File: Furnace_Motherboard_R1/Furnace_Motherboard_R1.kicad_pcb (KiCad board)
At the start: 2 copper layers, 13 parts, among them U1 STM32H563VITx

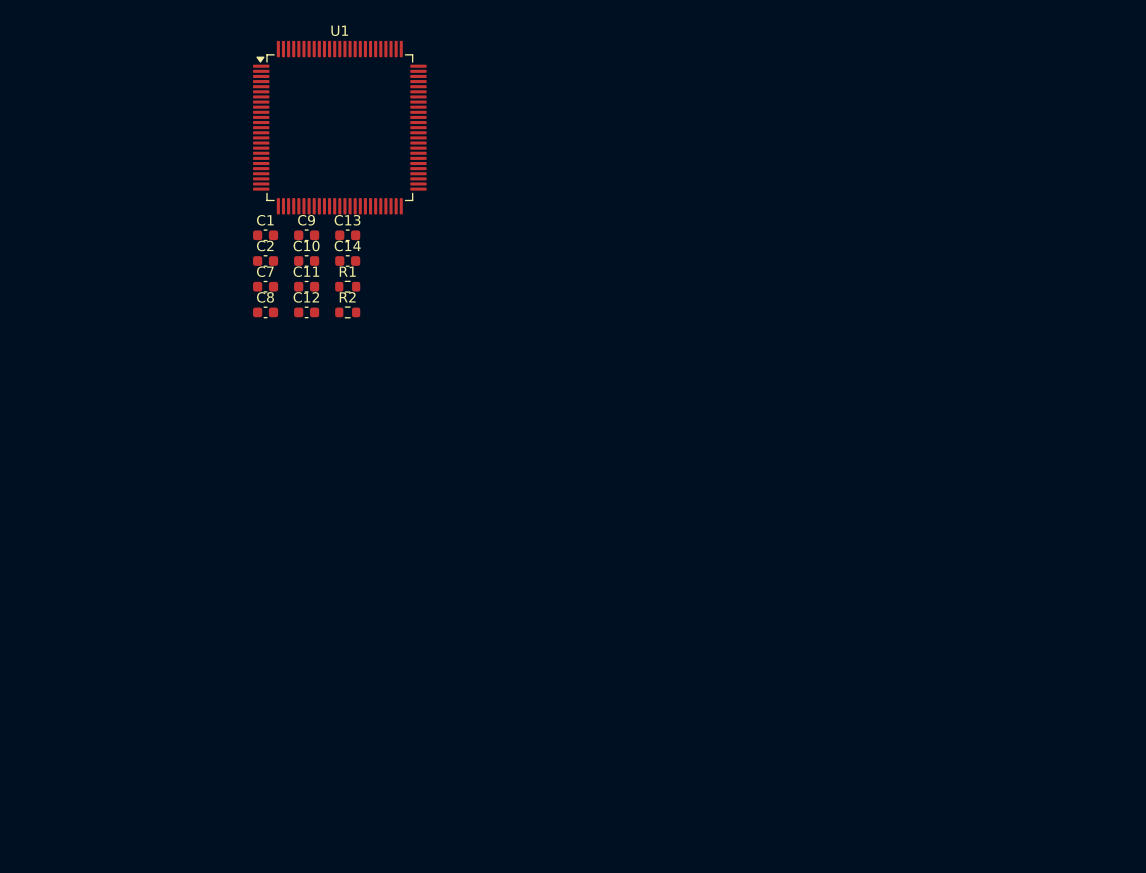
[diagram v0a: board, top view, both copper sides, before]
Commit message: Back up motherboard R1 design and fabrication outputs
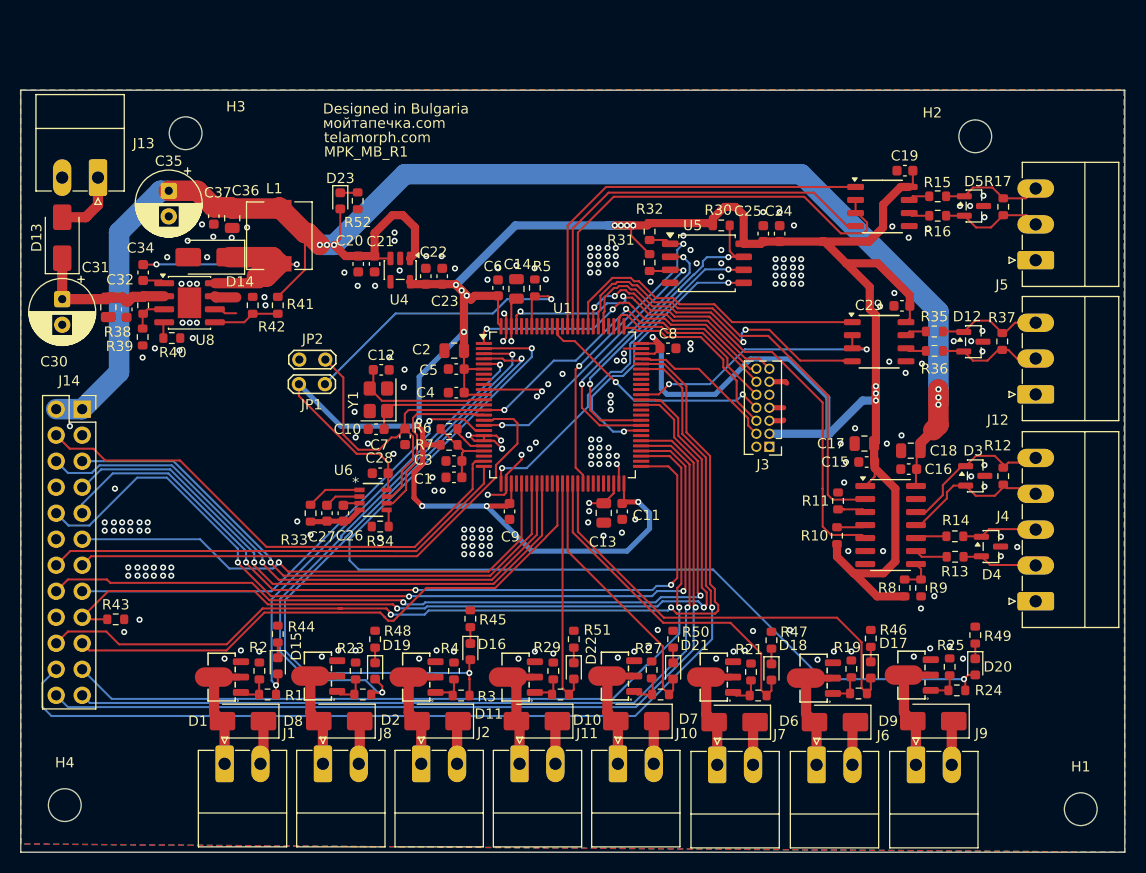
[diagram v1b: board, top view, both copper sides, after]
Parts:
- added C15: 100n, Capacitor_SMD:C_0603_1608Metric, F.Cu at (134.4, 93.1)
- added C16: 100n, Capacitor_SMD:C_0603_1608Metric, F.Cu at (138.5, 93.8)
- added C17: 1u, Capacitor_SMD:C_0805_2012Metric, F.Cu at (134.2, 91.3)
- added C18: 1u, Capacitor_SMD:C_0805_2012Metric, F.Cu at (138.7, 92.0)
- added C19: 100n, Capacitor_SMD:C_0603_1608Metric, F.Cu at (138.1, 64.7)
- added C20: 1u, Capacitor_SMD:C_0603_1608Metric, F.Cu at (84.8, 73.8)
- added C21: 100n, Capacitor_SMD:C_0603_1608Metric, F.Cu at (86.3, 73.8)
- added C22: 100n, Capacitor_SMD:C_0603_1608Metric, F.Cu at (91.3, 75.0)
- added C23: 1u, Capacitor_SMD:C_0603_1608Metric, F.Cu at (93.0, 75.0)
- added C24: 1u, Capacitor_SMD:C_0603_1608Metric, F.Cu at (125.9, 70.8)
- added C25: 100n, Capacitor_SMD:C_0603_1608Metric, F.Cu at (124.3, 70.8)
- added C26: 22n, Capacitor_SMD:C_0603_1608Metric, F.Cu at (83.3, 98.1)
- added C27: 3.3n, Capacitor_SMD:C_0603_1608Metric, F.Cu at (81.7, 98.1)
- added C28: 100n, Capacitor_SMD:C_0603_1608Metric, F.Cu at (86.9, 94.2)
- added C29: 100n, Capacitor_SMD:C_0603_1608Metric, F.Cu at (137.8, 77.9)
- added C3: 1u, Capacitor_SMD:C_0603_1608Metric, F.Cu at (94.1, 93.0)
- added C30: 47u, Capacitor_THT:CP_Radial_D6.3mm_P2.50mm, F.Cu at (55.9, 77.2)
- added C31: 2.2u, Capacitor_SMD:C_0805_2012Metric, F.Cu at (60.4, 78.0)
- added C32: 100n, Capacitor_SMD:C_0603_1608Metric, F.Cu at (62.1, 78.2)
- added C34: 100n, Capacitor_SMD:C_0603_1608Metric, F.Cu at (63.8, 74.6)
- added C35: 47u, Capacitor_THT:CP_Radial_D6.3mm_P2.50mm, F.Cu at (66.2, 66.6)
- added C36: 10u, Capacitor_SMD:C_0805_2012Metric, F.Cu at (72.5, 69.3)
- added C37: 100n, Capacitor_SMD:C_0603_1608Metric, F.Cu at (70.7, 69.1)
- added C4: 100n, Capacitor_SMD:C_0603_1608Metric, F.Cu at (94.3, 86.3)
- added C5: 100n, Capacitor_SMD:C_0603_1608Metric, F.Cu at (94.3, 84.0)
- added C6: 100n, Capacitor_SMD:C_0603_1608Metric, F.Cu at (98.4, 76.1)
- added D1: US1B, Diode_SMD:D_SMA, F.Cu at (73.5, 118.4)
- added D10: US1B, Diode_SMD:D_SMA, F.Cu at (111.9, 118.4)
- added D11: US1B, Diode_SMD:D_SMA, F.Cu at (102.2, 118.4)
- added D12: SM712_SOT23, Package_TO_SOT_SMD:SOT-23, F.Cu at (144.8, 81.4)
- added D13: SS36, Diode_SMD:D_SMA, F.Cu at (55.9, 71.2)
- added D14: SS36, Diode_SMD:D_SMA, F.Cu at (70.2, 73.1)
- added D15: LED, LED_SMD:LED_0603_1608Metric, F.Cu at (76.9, 113.0)
- added D16: LED, LED_SMD:LED_0603_1608Metric, F.Cu at (95.7, 111.6)
- added D17: LED, LED_SMD:LED_0603_1608Metric, F.Cu at (134.8, 113.4)
- added D18: LED, LED_SMD:LED_0603_1608Metric, F.Cu at (125.1, 113.6)
- added D19: LED, LED_SMD:LED_0603_1608Metric, F.Cu at (86.4, 113.5)
- added D2: US1B, Diode_SMD:D_SMA, F.Cu at (92.5, 118.4)
- added D20: LED, LED_SMD:LED_0603_1608Metric, F.Cu at (145.0, 113.1)
- added D21: LED, LED_SMD:LED_0603_1608Metric, F.Cu at (115.5, 113.5)
- added D22: LED, LED_SMD:LED_0603_1608Metric, F.Cu at (105.8, 113.5)
- added D23: LED, LED_SMD:LED_0603_1608Metric, F.Cu at (83.0, 67.6)
- added D3: SM712_SOT23, Package_TO_SOT_SMD:SOT-23, F.Cu at (145.0, 94.5)
- added D4: SM712_SOT23, Package_TO_SOT_SMD:SOT-23, F.Cu at (146.5, 101.4)
- added D5: SM712_SOT23, Package_TO_SOT_SMD:SOT-23, F.Cu at (144.9, 68.1)
- added D6: US1B, Diode_SMD:D_SMA, F.Cu at (131.3, 118.5)
- added D7: US1B, Diode_SMD:D_SMA, F.Cu at (121.5, 118.5)
- added D8: US1B, Diode_SMD:D_SMA, F.Cu at (82.9, 118.4)
- added D9: US1B, Diode_SMD:D_SMA, F.Cu at (140.9, 118.4)
- added H1: MountingHole, MountingHole:MountingHole_3.2mm_M3, F.Cu at (155.3, 127.0)
- added H2: MountingHole, MountingHole:MountingHole_3.2mm_M3, F.Cu at (145.0, 61.3)
- added H3: MountingHole, MountingHole:MountingHole_3.2mm_M3, F.Cu at (67.9, 61.0)
- added H4: MountingHole, MountingHole:MountingHole_3.2mm_M3, F.Cu at (56.1, 126.6)
- added J1: Conn_01x02, Connector_Phoenix_MC:PhoenixContact_MC_1,5_2-G-3.5_1x02_P3.50mm_Horizontal, F.Cu at (71.7, 122.6)
- added J10: Conn_01x02, Connector_Phoenix_MC:PhoenixContact_MC_1,5_2-G-3.5_1x02_P3.50mm_Horizontal, F.Cu at (110.1, 122.6)
- added J11: Conn_01x02, Connector_Phoenix_MC:PhoenixContact_MC_1,5_2-G-3.5_1x02_P3.50mm_Horizontal, F.Cu at (100.5, 122.6)
- added J12: Conn_01x03, Connector_Phoenix_MC:PhoenixContact_MC_1,5_3-G-3.5_1x03_P3.50mm_Horizontal, F.Cu at (150.9, 86.5)
- added J13: Conn_01x02, Connector_Phoenix_MC:PhoenixContact_MC_1,5_2-G-3.5_1x02_P3.50mm_Horizontal, F.Cu at (59.3, 65.3)
- added J14: Conn_02x12_Odd_Even, Connector_PinSocket_2.54mm:PinSocket_2x12_P2.54mm_Vertical, F.Cu at (57.8, 87.9)
- added J2: Conn_01x02, Connector_Phoenix_MC:PhoenixContact_MC_1,5_2-G-3.5_1x02_P3.50mm_Horizontal, F.Cu at (90.9, 122.6)
- added J3: Conn_02x07_Odd_Even, Connector_PinHeader_1.27mm:PinHeader_2x07_P1.27mm_Vertical, F.Cu at (124.9, 91.6)
- added J4: Conn_01x05, Connector_Phoenix_MC:PhoenixContact_MC_1,5_5-G-3.5_1x05_P3.50mm_Horizontal, F.Cu at (150.9, 106.7)
- added J5: Conn_01x03, Connector_Phoenix_MC:PhoenixContact_MC_1,5_3-G-3.5_1x03_P3.50mm_Horizontal, F.Cu at (150.9, 73.4)
- added J6: Conn_01x02, Connector_Phoenix_MC:PhoenixContact_MC_1,5_2-G-3.5_1x02_P3.50mm_Horizontal, F.Cu at (129.5, 122.7)
- added J7: Conn_01x02, Connector_Phoenix_MC:PhoenixContact_MC_1,5_2-G-3.5_1x02_P3.50mm_Horizontal, F.Cu at (119.8, 122.7)
- added J8: Conn_01x02, Connector_Phoenix_MC:PhoenixContact_MC_1,5_2-G-3.5_1x02_P3.50mm_Horizontal, F.Cu at (81.3, 122.6)
- added J9: Conn_01x02, Connector_Phoenix_MC:PhoenixContact_MC_1,5_2-G-3.5_1x02_P3.50mm_Horizontal, F.Cu at (139.2, 122.7)
- added JP1: Jumper_2_Open, TestPoint:TestPoint_2Pads_Pitch2.54mm_Drill0.8mm, F.Cu at (81.5, 85.5)
- added JP2: Jumper_2_Open, TestPoint:TestPoint_2Pads_Pitch2.54mm_Drill0.8mm, F.Cu at (79.0, 83.1)
- added L1: 33u, Inductor_SMD:L_6.3x6.3_H3, F.Cu at (77.0, 71.0)
- added Q1: BSS606N, PCM_JLCPCB:Q_SOT-89, F.Cu at (72.0, 114.1)
- added Q2: BSS606N, PCM_JLCPCB:Q_SOT-89, F.Cu at (91.0, 114.1)
- added Q3: BSS606N, PCM_JLCPCB:Q_SOT-89, F.Cu at (129.8, 114.2)
- added Q4: BSS606N, PCM_JLCPCB:Q_SOT-89, F.Cu at (120.0, 114.1)
- added Q5: BSS606N, PCM_JLCPCB:Q_SOT-89, F.Cu at (81.4, 114.0)
- added Q6: BSS606N, PCM_JLCPCB:Q_SOT-89, F.Cu at (139.3, 113.9)
- added Q7: BSS606N, PCM_JLCPCB:Q_SOT-89, F.Cu at (110.4, 114.0)
- added Q8: BSS606N, PCM_JLCPCB:Q_SOT-89, F.Cu at (100.7, 114.1)
- added R10: 10k, Resistor_SMD:R_0603_1608Metric, F.Cu at (131.5, 100.3)
- added R11: 10k, Resistor_SMD:R_0603_1608Metric, F.Cu at (131.6, 96.9)
- added R12: 120, Resistor_SMD:R_0603_1608Metric, F.Cu at (147.7, 94.5)
- added R13: 15, Resistor_SMD:R_0603_1608Metric, F.Cu at (143.0, 102.4)
- added R14: 15, Resistor_SMD:R_0603_1608Metric, F.Cu at (143.0, 100.4)
- added R15: 15, Resistor_SMD:R_0603_1608Metric, F.Cu at (141.3, 67.2)
- added R16: 15, Resistor_SMD:R_0603_1608Metric, F.Cu at (141.3, 69.1)
- added R17: 120, Resistor_SMD:R_0603_1608Metric, F.Cu at (147.7, 68.2)
- added R18: 100, Resistor_SMD:R_0603_1608Metric, F.Cu at (133.6, 115.7)
- added R19: 10k, Resistor_SMD:R_0603_1608Metric, F.Cu at (132.9, 113.3)
- added R20: 100, Resistor_SMD:R_0603_1608Metric, F.Cu at (123.8, 115.9)
- added R21: 10k, Resistor_SMD:R_0603_1608Metric, F.Cu at (123.1, 113.6)
- added R22: 100, Resistor_SMD:R_0603_1608Metric, F.Cu at (85.2, 115.8)
- added R23: 10k, Resistor_SMD:R_0603_1608Metric, F.Cu at (84.5, 113.5)
- added R24: 100, Resistor_SMD:R_0603_1608Metric, F.Cu at (143.2, 115.4)
- added R25: 10k, Resistor_SMD:R_0603_1608Metric, F.Cu at (142.5, 113.1)
- added R26: 100, Resistor_SMD:R_0603_1608Metric, F.Cu at (114.3, 115.8)
- added R27: 10k, Resistor_SMD:R_0603_1608Metric, F.Cu at (113.4, 113.4)
- added R28: 100, Resistor_SMD:R_0603_1608Metric, F.Cu at (104.5, 115.8)
- added R29: 10k, Resistor_SMD:R_0603_1608Metric, F.Cu at (103.8, 113.5)
- added R3: 100, Resistor_SMD:R_0603_1608Metric, F.Cu at (94.8, 115.9)
- added R30: 10k, Resistor_SMD:R_0603_1608Metric, F.Cu at (120.2, 70.0)
- added R31: 10k, Resistor_SMD:R_0603_1608Metric, F.Cu at (113.2, 73.6)
- added R32: 10k, Resistor_SMD:R_0603_1608Metric, F.Cu at (113.2, 70.6)
- added R33: 10k, Resistor_SMD:R_0603_1608Metric, F.Cu at (80.1, 98.1)
- added R34: 10k, Resistor_SMD:R_0603_1608Metric, F.Cu at (86.9, 99.4)
- added R35: 15, Resistor_SMD:R_0603_1608Metric, F.Cu at (141.0, 80.4)
- added R36: 15, Resistor_SMD:R_0603_1608Metric, F.Cu at (141.0, 82.3)
- added R37: 120, Resistor_SMD:R_0603_1608Metric, F.Cu at (147.6, 81.3)
- added R38: 560k, Resistor_SMD:R_0603_1608Metric, F.Cu at (63.8, 77.8)
- added R39: 39k, Resistor_SMD:R_0603_1608Metric, F.Cu at (63.7, 80.9)
- added R4: 10k, Resistor_SMD:R_0603_1608Metric, F.Cu at (94.1, 113.5)
- added R40: 56k, Resistor_SMD:R_0603_1608Metric, F.Cu at (66.5, 81.0)
- added R41: 56k, Resistor_SMD:R_0603_1608Metric, F.Cu at (76.9, 77.8)
- added R42: 10k, Resistor_SMD:R_0603_1608Metric, F.Cu at (74.5, 77.8)
- added R43: 10k, Resistor_SMD:R_0603_1608Metric, F.Cu at (61.1, 108.5)
- added R44: 150, Resistor_SMD:R_0603_1608Metric, F.Cu at (76.9, 109.9)
- added R45: 150, Resistor_SMD:R_0603_1608Metric, F.Cu at (95.7, 108.4)
- added R46: 150, Resistor_SMD:R_0603_1608Metric, F.Cu at (134.8, 110.3)
- added R47: 150, Resistor_SMD:R_0603_1608Metric, F.Cu at (125.1, 110.5)
- added R48: 150, Resistor_SMD:R_0603_1608Metric, F.Cu at (86.4, 110.4)
- added R49: 150, Resistor_SMD:R_0603_1608Metric, F.Cu at (145.0, 110.0)
- added R5: 10k, Resistor_SMD:R_0603_1608Metric, F.Cu at (102.0, 76.1)
- added R50: 150, Resistor_SMD:R_0603_1608Metric, F.Cu at (115.5, 110.4)
- added R51: 150, Resistor_SMD:R_0603_1608Metric, F.Cu at (105.8, 110.4)
- added R52: 330, Resistor_SMD:R_0603_1608Metric, F.Cu at (84.7, 67.6)
- added R6: 0, Resistor_SMD:R_0603_1608Metric, F.Cu at (93.6, 89.9)
- added R7: 0, Resistor_SMD:R_0603_1608Metric, F.Cu at (93.6, 91.4)
- added R8: 10k, Resistor_SMD:R_0603_1608Metric, F.Cu at (138.1, 105.4)
- added R9: 0, Resistor_SMD:R_0603_1608Metric, F.Cu at (139.7, 105.4)
- added U2: PTHVD2452VDR, PCM_JLCPCB:SOIC-14_L8.7-W3.9-P1.27-LS6.0-BL, F.Cu at (136.7, 99.3)
- added U3: THVD2450DR, PCM_JLCPCB:SOIC-8_3.9x4.9mm_P1.27mm, F.Cu at (135.9, 68.2)
- added U4: TPS7A20xxxDBV, Package_TO_SOT_SMD:SOT-23-5, F.Cu at (88.8, 74.4)
- added U5: W25Q128JVS, Package_SO:SOIC-8_5.3x5.3mm_P1.27mm, F.Cu at (118.8, 73.7)
- added U6: TPS36BA38ACADDFRQ1, Furnace_TI:SOT-23-THIN-8_DDF_TEX, F.Cu at (86.2, 96.8)
- added U7: THVD2450DR, PCM_JLCPCB:SOIC-8_3.9x4.9mm_P1.27mm, F.Cu at (135.6, 81.4)
- added U8: LMR16030SDDAR, Package_SO:SOIC-8-1EP_3.9x4.9mm_P1.27mm_EP2.29x3mm, F.Cu at (68.3, 77.5)
- added Y1: Crystal_GND24_Small, Crystal:Crystal_SMD_3225-4Pin_3.2x2.5mm, F.Cu at (86.7, 87.0)
- C1: value 2.2u -> 100n
- C10: value 100n -> C
- C12: value 1u -> C
- C13: value 100n -> 2.2u; footprint Capacitor_SMD:C_0603_1608Metric -> Capacitor_SMD:C_0805_2012Metric
- C14: value 4.7u -> 2.2u; footprint Capacitor_SMD:C_0603_1608Metric -> Capacitor_SMD:C_0805_2012Metric
- C2: value 2.2u -> 4.7u; footprint Capacitor_SMD:C_0603_1608Metric -> Capacitor_SMD:C_0805_2012Metric
- R1: value 0 -> 100
- R2: value 0 -> 10k
- moved R1 40.6 mm to (75.9, 115.8), turned to 180 degrees
- moved C8 39.5 mm to (115.0, 82.0)
- moved C11 37.8 mm to (110.5, 97.9), turned to -90 degrees
- moved C13 36.9 mm to (108.7, 98.1), turned to -90 degrees
- moved R2 36.1 mm to (75.1, 113.5), turned to 90 degrees
- moved U1 34.7 mm to (104.7, 87.5)
- moved C9 33.5 mm to (99.5, 97.9), turned to -90 degrees
- moved C1 29.9 mm to (94.1, 94.6), turned to 180 degrees
- moved C2 20.4 mm to (94.1, 82.2), turned to 180 degrees
- moved C7 20.0 mm to (89.3, 90.6), turned to -90 degrees
- moved C10 17.8 mm to (86.5, 89.9), turned to 180 degrees
- moved C14 16.7 mm to (100.2, 76.2), turned to 90 degrees
- moved C12 9.19 mm to (87.0, 84.1)
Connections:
- C1 pad 1: Net-(C1-Pad1) -> /MAIN_MCU/VDDA
- C1 pad 2: MCU_GND -> GND
- C10 pad 1: +3V3 -> /MAIN_MCU/RCC_OSC_OUT
- C10 pad 2: MCU_GND -> GND
- C11 pad 2: MCU_GND -> GND
- C12 pad 1: +3V3 -> /MAIN_MCU/RCC_OSC_IN
- C12 pad 2: MCU_GND -> GND
- C13 pad 1: +3V3 -> Net-(C13-Pad1)
- C13 pad 2: MCU_GND -> GND
- C14 pad 1: +3V3 -> Net-(C13-Pad1)
- C14 pad 2: MCU_GND -> GND
- C2 pad 1: Net-(C2-Pad1) -> +3V3
- C2 pad 2: MCU_GND -> GND
- C7 pad 1: +3V3 -> /SUP_RESET_N
- C7 pad 2: MCU_GND -> GND
- C8 pad 2: MCU_GND -> GND
- C9 pad 2: MCU_GND -> GND
- R1 pad 1: Net-(U1-VBAT) -> /AUX_DO3_CMD
- R1 pad 2: Net-(U1-VDDA) -> Net-(Q1-G)
- R2 pad 1: +3V3 -> Net-(Q1-G)
- R2 pad 2: Net-(U1-VREF+) -> GND
- U1 pad 1: unconnected-(U1-PE2-Pad1) -> /MAIN_MCU/UART8_TX
- U1 pad 10: MCU_GND -> GND
- U1 pad 100: Net-(U1-VBAT) -> +3V3
- U1 pad 11: Net-(U1-VBAT) -> +3V3
- U1 pad 12: unconnected-(U1-PH0-Pad12) -> /MAIN_MCU/RCC_OSC_IN
- U1 pad 13: unconnected-(U1-PH1-Pad13) -> /MAIN_MCU/RCC_OSC_OUT
- U1 pad 14: unconnected-(U1-NRST-Pad14) -> /SUP_RESET_N
- U1 pad 15: unconnected-(U1-PC0-Pad15) -> /SUP_WDI
- U1 pad 16: unconnected-(U1-PC1-Pad16) -> /ETH_MDC
- U1 pad 17: unconnected-(U1-PC2-Pad17) -> /OCTOSPI1_IO2
- U1 pad 18: unconnected-(U1-PC3-Pad18) -> /ETH_PHY_RST_N
- U1 pad 19: MCU_GND -> GND
- U1 pad 2: unconnected-(U1-PE3-Pad2) -> /AUX_DO0_CMD
- U1 pad 20: MCU_GND -> GND
- U1 pad 22: Net-(U1-VDDA) -> /MAIN_MCU/VDDA
- U1 pad 24: unconnected-(U1-PA1-Pad24) -> /ETH_REF_CLK
- U1 pad 25: unconnected-(U1-PA2-Pad25) -> /ETH_MDIO
- U1 pad 26: unconnected-(U1-PA3-Pad26) -> /OCTOSPI1_CLK
- U1 pad 27: MCU_GND -> GND
- U1 pad 28: Net-(U1-VBAT) -> +3V3
- U1 pad 3: unconnected-(U1-PE4-Pad3) -> /AUX_DO1_CMD
- U1 pad 30: unconnected-(U1-PA5-Pad30) -> /ETH_TX_EN
- U1 pad 32: unconnected-(U1-PA7-Pad32) -> /ETH_CRS_DV
- U1 pad 33: unconnected-(U1-PC4-Pad33) -> /ETH_RXD0
- U1 pad 34: unconnected-(U1-PC5-Pad34) -> /ETH_RXD1
- U1 pad 37: unconnected-(U1-PB2-Pad37) -> /CAN_STB
- U1 pad 38: unconnected-(U1-PE7-Pad38) -> /AUX_DO4_CMD
- U1 pad 39: unconnected-(U1-PE8-Pad39) -> /AUX_DO5_CMD
- U1 pad 4: unconnected-(U1-PE5-Pad4) -> /AUX_DO2_CMD
- U1 pad 40: unconnected-(U1-PE9-Pad40) -> /HEATER_CONTACTOR_CMD
- U1 pad 41: unconnected-(U1-PE10-Pad41) -> /HEATER_SSR_CMD
- U1 pad 42: unconnected-(U1-PE11-Pad42) -> /OCTOSPI1_NCS
- U1 pad 48: Net-(C1-Pad1) -> Net-(C13-Pad1)
- U1 pad 49: MCU_GND -> GND
- U1 pad 5: unconnected-(U1-PE6-Pad5) -> /AUX_DO3_CMD
- U1 pad 51: unconnected-(U1-PB12-Pad51) -> /ETH_TXD0
- U1 pad 53: unconnected-(U1-PB14-Pad53) -> /EXT_RS485_DE
- U1 pad 54: unconnected-(U1-PB15-Pad54) -> /ETH_TXD1
- U1 pad 55: unconnected-(U1-PD8-Pad55) -> /EXT_RS485_TX
- U1 pad 56: unconnected-(U1-PD9-Pad56) -> /EXT_RS485_RX
- U1 pad 58: unconnected-(U1-PD11-Pad58) -> /OCTOSPI1_IO0
- U1 pad 59: unconnected-(U1-PD12-Pad59) -> /OCTOSPI1_IO1
- U1 pad 6: Net-(U1-VBAT) -> +3V3
- U1 pad 60: unconnected-(U1-PD13-Pad60) -> /OCTOSPI1_IO3
- U1 pad 63: unconnected-(U1-PC6-Pad63) -> /ETH_PHY_INT_N
- U1 pad 64: unconnected-(U1-PC7-Pad64) -> /ETH_MODULE_PRESENT
- U1 pad 65: unconnected-(U1-PC8-Pad65) -> /AUX_RS485_DE
- U1 pad 70: unconnected-(U1-PA11-Pad70) -> /FDCAN1_RX
- U1 pad 71: unconnected-(U1-PA12-Pad71) -> /FDCAN1_TX
- U1 pad 72: unconnected-(U1-PA13(JTMS-Pad72) -> /MAIN_MCU/DEBUG_JTMS-SWDIO
- U1 pad 73: Net-(U1-VBAT) -> +3V3
- U1 pad 74: MCU_GND -> GND
- U1 pad 75: Net-(U1-VBAT) -> +3V3
- U1 pad 76: unconnected-(U1-PA14(JTCK-Pad76) -> /MAIN_MCU/DEBUG_JTCK-SWCLK
- U1 pad 77: unconnected-(U1-PA15(JTDI)-Pad77) -> /MAIN_MCU/DEBUG_JTDI
- U1 pad 80: unconnected-(U1-PC12-Pad80) -> /AUX_RS485_TX
- U1 pad 81: unconnected-(U1-PD0-Pad81) -> /RS422_RX
- U1 pad 82: unconnected-(U1-PD1-Pad82) -> /RS422_TX
- U1 pad 83: unconnected-(U1-PD2-Pad83) -> /AUX_RS485_RX
- U1 pad 85: unconnected-(U1-PD4-Pad85) -> /INT_RS485_DE
- U1 pad 86: unconnected-(U1-PD5-Pad86) -> /INT_RS485_TX
- U1 pad 87: unconnected-(U1-PD6-Pad87) -> /INT_RS485_RX
- U1 pad 89: unconnected-(U1-PB3(JTDO-Pad89) -> /MAIN_MCU/DEBUG_JTDO-SWO
- U1 pad 94: unconnected-(U1-BOOT0-Pad94) -> /MAIN_MCU/BOOT0
- U1 pad 97: unconnected-(U1-PE0-Pad97) -> /MAIN_MCU/UART8_RX
- U1 pad 98: Net-(C2-Pad1) -> Net-(C13-Pad1)
- U1 pad 99: MCU_GND -> GND
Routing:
- net +3V3: track 0.00 -> 286.6 mm, vias 0 -> 16
- net +5V: track 0.00 -> 160.9 mm, vias 0 -> 6
- net /FDCAN1_RX: track 0.00 -> 103.6 mm, vias 0 -> 1
- net /AUX_DO0_CMD: track 0.00 -> 100.0 mm, vias 0 -> 2
- net /FDCAN1_TX: track 0.00 -> 97.0 mm, vias 0 -> 2
- net /ETH_MODULE_PRESENT: track 0.00 -> 89.8 mm, vias 0 -> 2
- net /EXT_RS485_RX: track 0.00 -> 89.5 mm, vias 0 -> 1
- net /ETH_PHY_INT_N: track 0.00 -> 86.8 mm, vias 0 -> 2
- net /ETH_TXD1: track 0.00 -> 86.7 mm, vias 0 -> 3
- net /EXT_RS485_TX: track 0.00 -> 85.2 mm, vias 0 -> 1
- net /EXT_RS485_DE: track 0.00 -> 83.0 mm, vias 0 -> 1
- net /ETH_TXD0: track 0.00 -> 80.1 mm, vias 0 -> 3
- net /SUP_RESET_N: track 0.00 -> 67.0 mm, vias 0 -> 2
- net /AUX_DO2_CMD: track 0.00 -> 64.4 mm, vias 0 -> 2
- net /ETH_RXD0: track 0.00 -> 59.6 mm, vias 0 -> 1
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- added copper zone on B.Cu, net GND
- added copper zone on F.Cu, net GND
- added copper zone on In1.Cu, net GND
- added copper zone on In2.Cu, net GND
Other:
- board outline added: 107.8 x 74.4 mm
- copper layers 2 -> 4
- board text added: "Designed in Bulgaria"
- board text added: "MPK_MB_R1"
- board text added: "telamorph.com"
- board text added: "мойтапечка.com"
